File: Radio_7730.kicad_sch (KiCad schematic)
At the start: 1 part

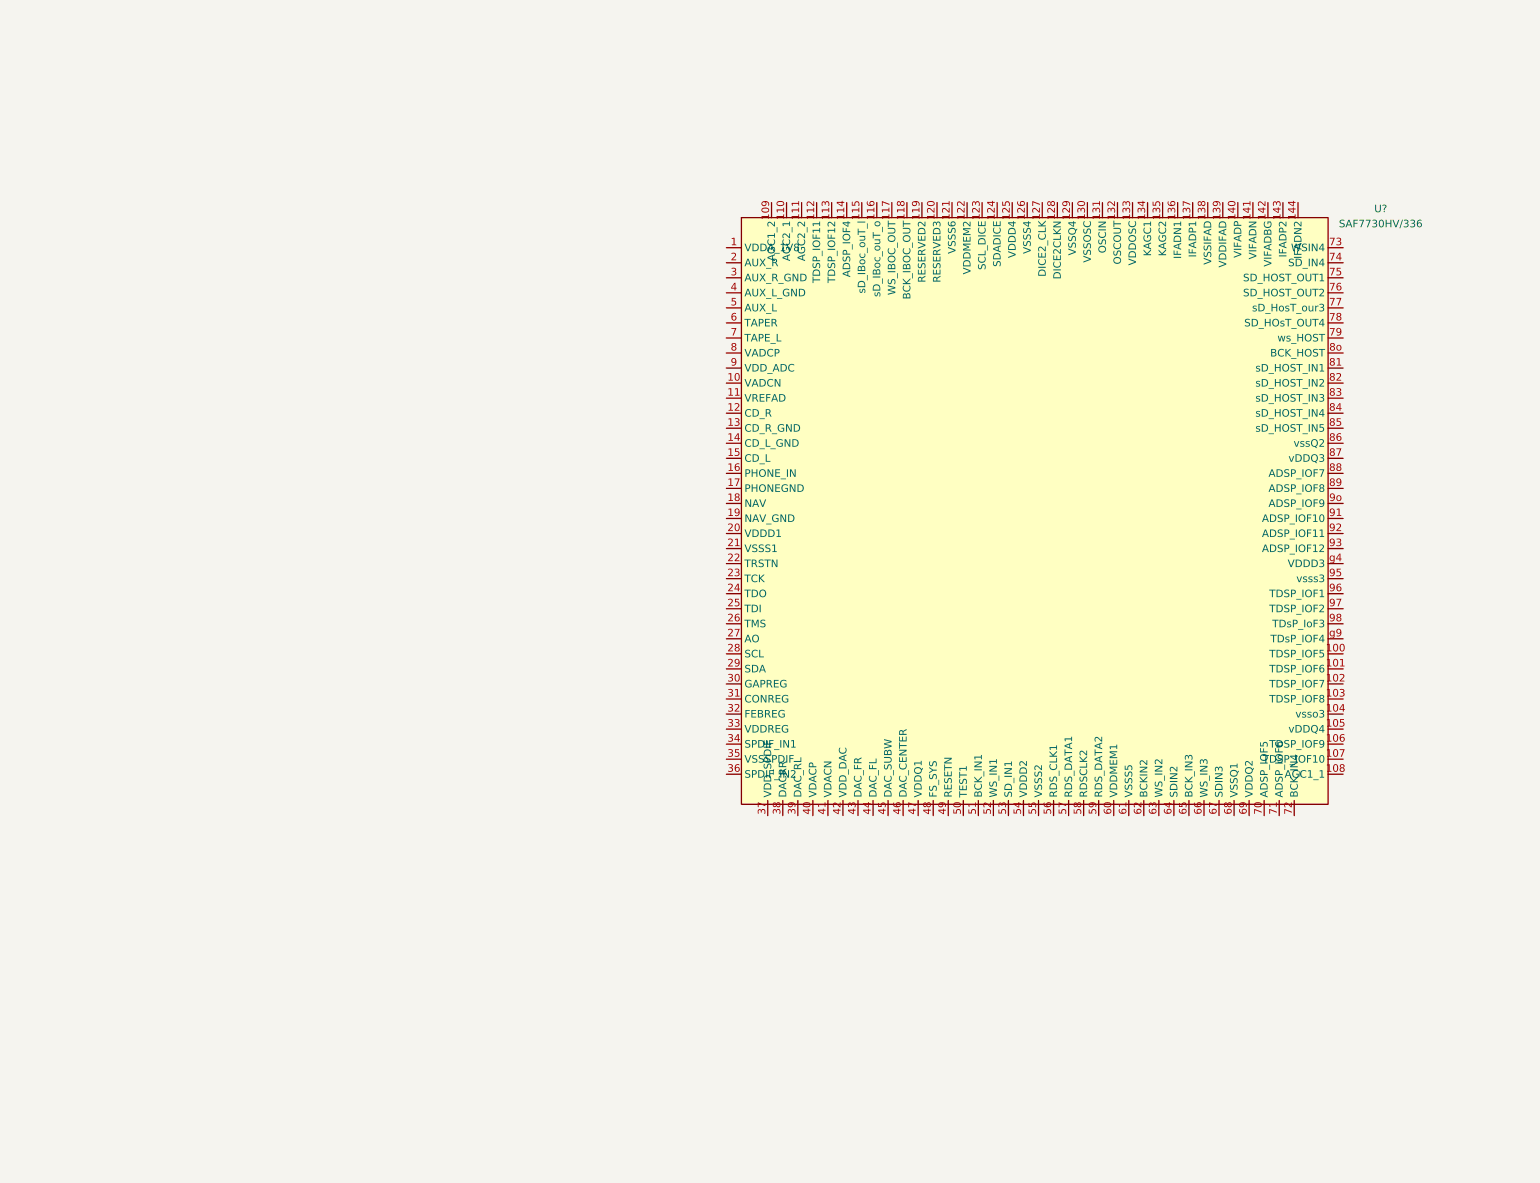
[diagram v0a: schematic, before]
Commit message: Finish SAF7730 routing
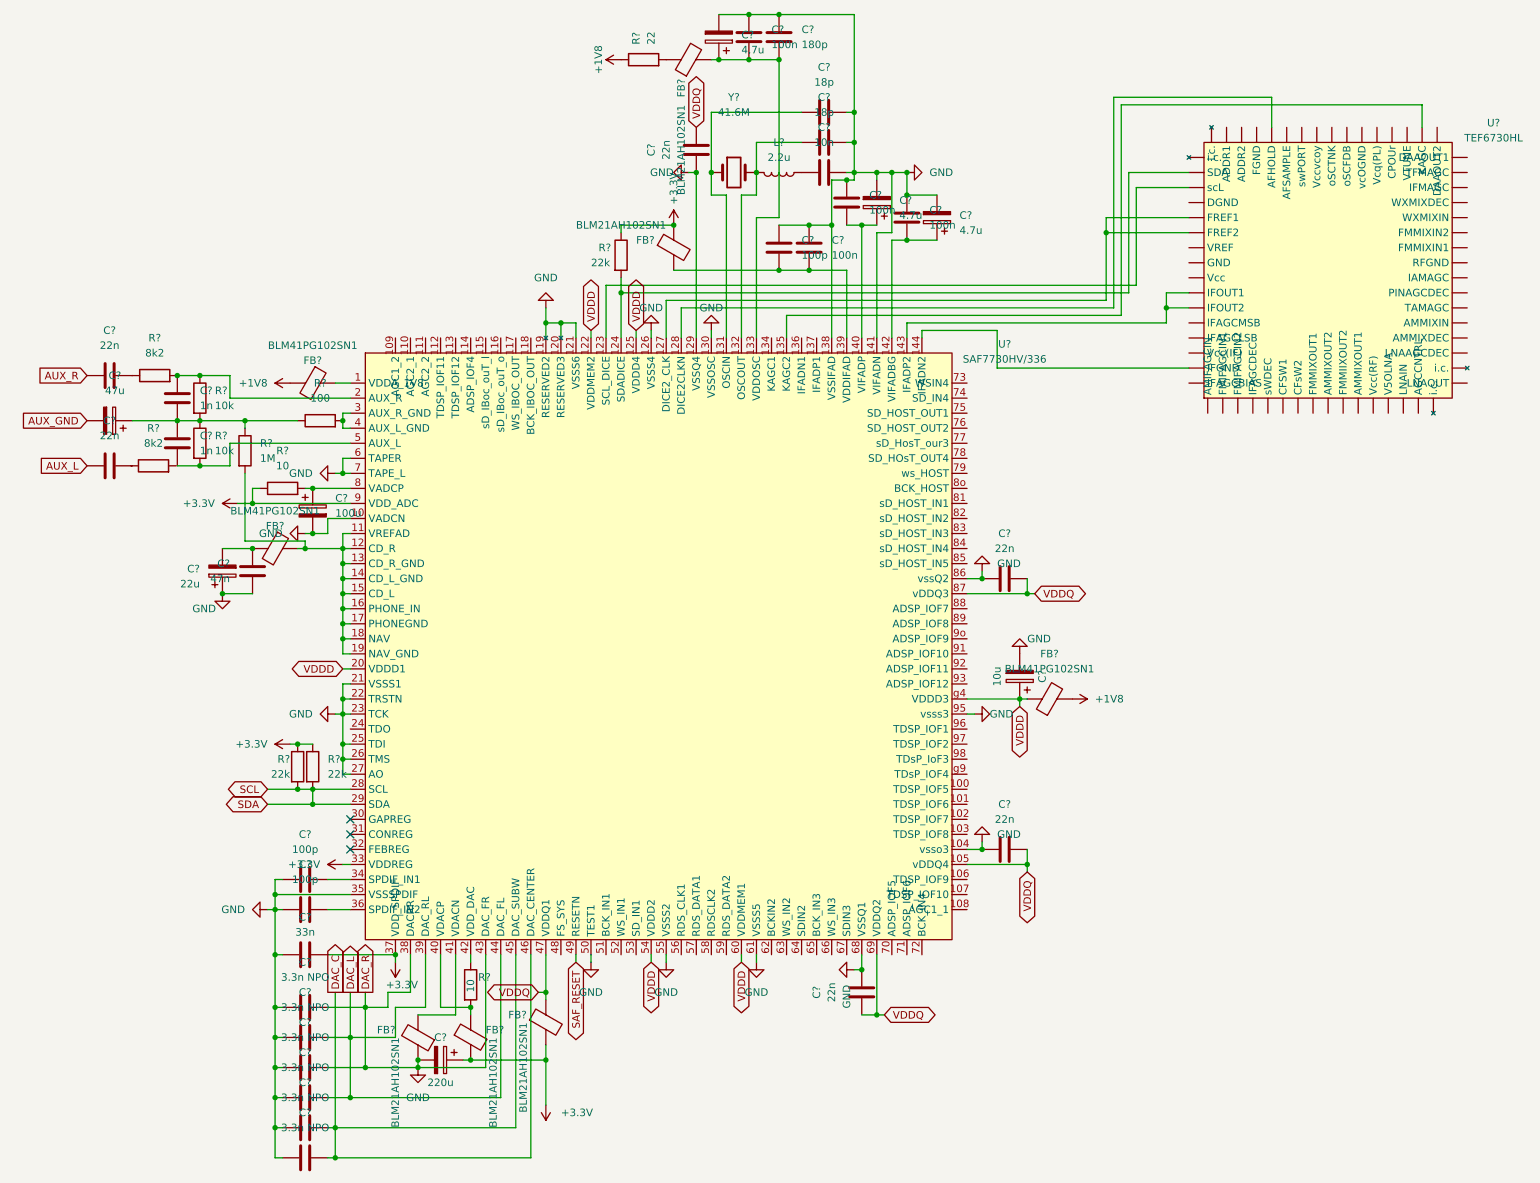
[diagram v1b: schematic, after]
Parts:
- removed U?: SAF7730HV/336, symbol NXP_Radio:SAF7730HV/336
- added C? (x2): 18p, symbol Device:C
- added C? (x3): 4.7u, symbol Device:C_Polarized
- added C? (x6): 3.3n NPO, symbol Device:C
- added C? (x3): 100p, symbol Device:C
- added C? (x6): 22n, symbol Device:C
- added C?: 100u, symbol Device:C_Polarized
- added C?: 180p, symbol Device:C
- added C?: 47n, symbol Device:C
- added C? (x4): 100n, symbol Device:C
- added C?: 47u, symbol Device:C_Polarized
- added C?: 10u, symbol Device:C_Polarized
- added C?: 220u, symbol Device:C_Polarized
- added C?: 10n, symbol Device:C
- added C? (x2): 1n, symbol Device:C
- added C?: 22u, symbol Device:C_Polarized
- added C?: 33n, symbol Device:C
- added FB? (x5): BLM21AH102SN1, symbol Device:FerriteBead
- added FB? (x3): BLM41PG102SN1, symbol Device:FerriteBead
- added L?: 2.2u, symbol Device:L
- added R? (x2): 10, symbol Device:R
- added R? (x2): 10k, symbol Device:R
- added R? (x2): 8k2, symbol Device:R
- added R? (x3): 22k, symbol Device:R
- added R?: 100, symbol Device:R
- added R?: 22, symbol Device:R
- added R?: 1M, symbol Device:R
- added U?: TEF6730HL, symbol NXP_Radio:TEF6730HL
- added U?: SAF7730HV/336, symbol NXP_Radio:SAF7730HV/336
- added Y?: 41.6M, symbol Device:Crystal
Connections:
- new net: FB?.1, R?.2, U?.40 (VDACP)
- new net: C?.2, L?.2, U?.132 (OSCOUT), Y?.2
- new net: C?.1, C?.2, U?.142 (VIFADBG)
- new net: FB?.2, U?.41 (VDACN)
- new net: C?.1, R?.2, U?.8 (VADCP)
- new net: C?.1, U?.131 (OSCIN), Y?.1
- new net: C?.2, U?.34 (SPDIF_IN1)
- new net: U?. (WXMIXIN), U?.123 (SCL_DICE)
- new net: R?.2, U?. (WXMIXIN), U?.124 (SDADICE)
- new net: U?. (WXMIXIN), U?.127 (DICE2_CLK)
- new net: U?. (WXMIXIN), U?.128 (DICE2CLKN)
- new net: U?. (WXMIXIN), U?.135 (KAGC2)
- new net: U?. (WXMIXIN), U?.143 (IFADP2)
- new net: U?. (WXMIXIN), U?.144 (IFADN2)
- new net: C?.2, U?.36 (SPDIF_IN2)
- new net: FB?.1, R?.2
- new net: C?.1, C?.2, C?.2, FB?.2, U?.133 (VDDOSC)
- new net: C?.1, C?.2, U?.140 (VIFADP)
- new net: FB?.1, U?.1 (VDDA_1V8)
- new net: FB?.1, R?.2, U?.11 (VREFAD), U?.12 (CD_R), U?.13 (CD_R_GND), U?.14 (CD_L_GND), U?.15 (CD_L), U?.16 (PHONE_IN), U?.17 (PHONEGND), U?.18 (NAV), U?.19 (NAV_GND)
- new net: C?.2, C?.2, FB?.2, U?.139 (VDDIFAD)
- new net: C?.1, R?.1, R?.2, U?.2 (AUX_R)
- new net: R?.2, U?.3 (AUX_R_GND), U?.4 (AUX_L_GND)
- new net: R?.1, U?.42 (VDD_DAC)
- new net: C?.2, R?.2, U?.5 (AUX_L)
- new net: C?.1, C?.1, C?.2, R?.1, R?.1, R?.1, R?.2
- new net: C?.1, C?.2, FB?.2
- new net: C?.1, L?.1
- new net: C?.2, R?.1
- new net +1V8: FB?.2, FB?.2, R?.1
- new net +3V3: C?.1, C?.2, FB?.1, FB?.2, FB?.2, R?.1, R?.1, R?.1, R?.1, U?.33 (VDDREG), U?.37 (VDD_SPDIF), U?.9 (VDD_ADC)
- new net AUX_GND: C?.2
- new net AUX_L: C?.1
- new net AUX_R: C?.1
- new net DAC_C: C?.2, C?.2, U?.45 (DAC_SUBW), U?.46 (DAC_CENTER)
- new net DAC_L: C?.2, C?.2, U?.39 (DAC_RL), U?.44 (DAC_FL)
- new net GND: C?.1, C?.1, C?.1, C?.1, C?.1, C?.1, C?.1, C?.1, C?.1, C?.1, C?.1, C?.1, C?.1, C?.1, C?.1, C?.1, C?.1, C?.1, C?.1, C?.1, C?.1, C?.2, C?.2, C?.2, C?.2, C?.2, C?.2, C?.2, C?.2, C?.2, C?.2, C?.2, FB?.1, U?.10 (VADCN), U?.104 (vsso3), U?.119 (RESERVED2), U?.120 (RESERVED3), U?.121 (VSSS6), U?.126 (VSSS4), U?.129 (VSSQ4), U?.130 (VSSOSC), U?.138 (VSSIFAD), U?.141 (VIFADN), U?.21 (VSSS1), U?.22 (TRSTN), U?.23 (TCK), U?.25 (TDI), U?.26 (TMS), U?.27 (AO), U?.35 (VSSSPDIF), U?.38 (DACRR), U?.43 (DAC_FR), U?.50 (TEST1), U?.55 (VSSS2), U?.6 (TAPER), U?.61 (VSSS5), U?.68 (VSSQ1), U?.7 (TAPE_L), U?.86 (vssQ2), U?.95 (vsss3)
- new net SAF_RESET: U?.49 (RESETN)
- new net SCL: R?.2, R?.2, U?.28 (SCL), U?.29 (SDA)
- new net VDDD: C?.1, FB?.1, U?.122 (VDDMEM2), U?.125 (VDDD4), U?.20 (VDDD1), U?.54 (VDDD2), U?.60 (VDDMEM1), U?.g4 (VDDD3)
- new net VDDQ: C?.2, C?.2, C?.2, C?.2, FB?.1, U?.105 (vDDQ4), U?.47 (VDDQ1), U?.69 (VDDQ2), U?.87 (vDDQ3)
- no-connect marks 0 -> 3
